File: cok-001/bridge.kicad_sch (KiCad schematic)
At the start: 40 parts, among them U7301 CXD9208GP

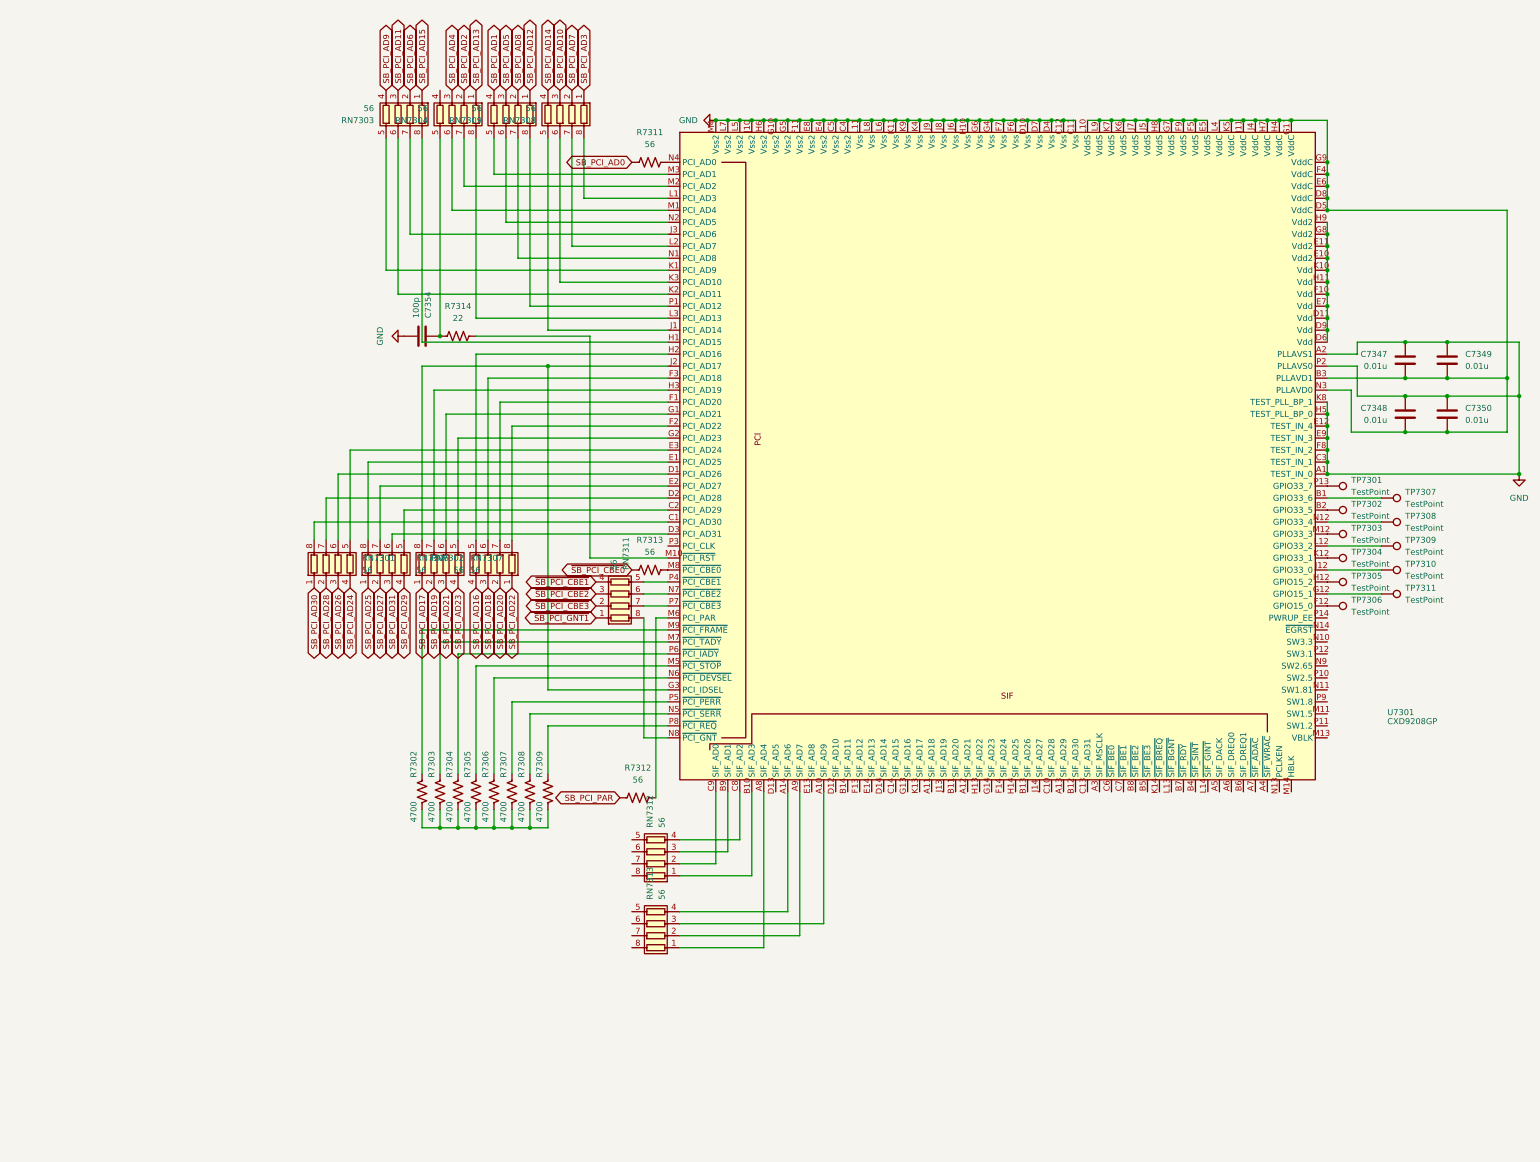
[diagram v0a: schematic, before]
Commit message: add some stupid n channel mosfet
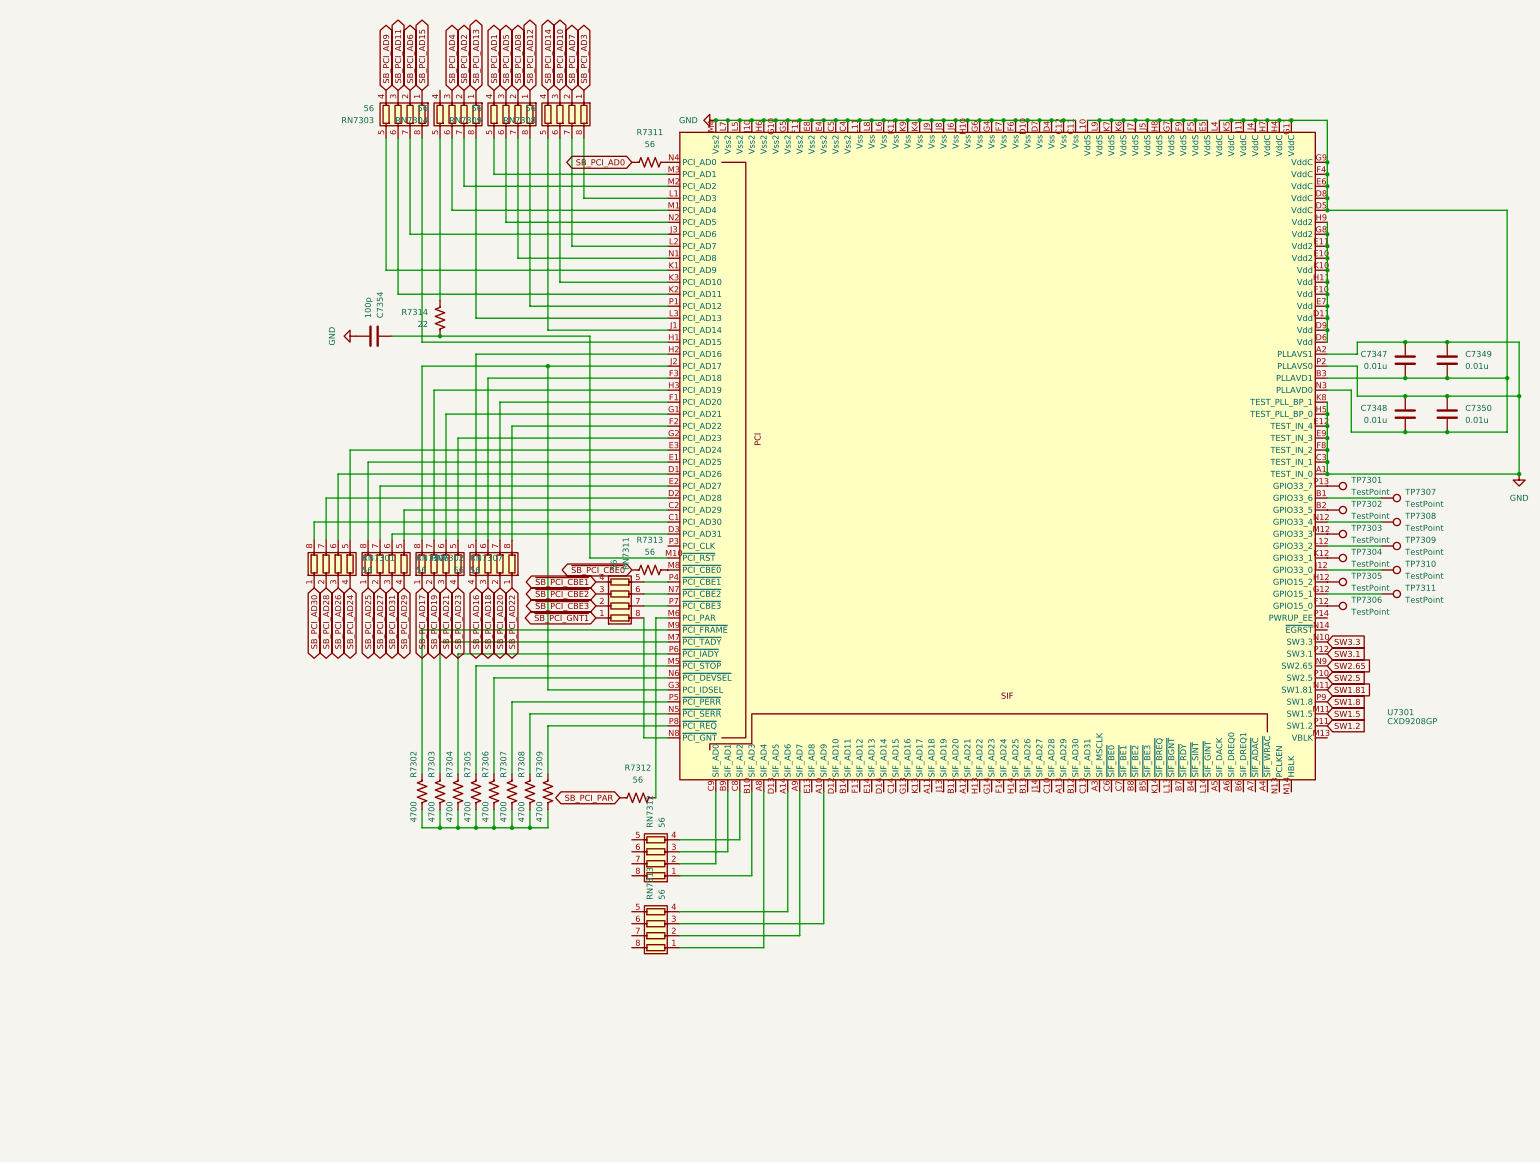
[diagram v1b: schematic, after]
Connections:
- net at C7354.1, R7314.1: now also U7301.M10 (~{PCI_RST}); no longer RN7304.5 (R4.2)
- net at R7314.2: now also RN7304.5 (R4.2); no longer U7301.M10 (~{PCI_RST})
- net SW1.5: now reaches U7301.M11 (SW1.5)
- net SW3.3: now reaches U7301.N10 (SW3.3)
- net SW1.81: now reaches U7301.N11 (SW1.81)
- net SW2.65: now reaches U7301.N9 (SW2.65)
- net SW2.5: now reaches U7301.P10 (SW2.5)
- net SW1.2: now reaches U7301.P11 (SW1.2)
- net SW3.1: now reaches U7301.P12 (SW3.1)
- net SW1.8: now reaches U7301.P9 (SW1.8)
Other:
- moved on the sheet: C7354, R7314
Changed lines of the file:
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@@
 	)
 	(junction
+		(at 48.26 69.85)
+		(diameter 0)
+		(color 0 0 0 0)
+	)
+	(junction
 		(at 152.4 24.13)
 		(diameter 0)
@@
 	)
 	(junction
-		(at 48.26 69.85)
-		(diameter 0)
-		(color 0 0 0 0)
-	)
-	(junction
 		(at 165.1 24.13)
 		(diameter 0)
@@
 	(wire
 		(pts
+			(xy 48.26 62.23) (xy 48.26 27.94)
+		)
+		(stroke
+			(width 0)
+			(type default)
+		)
+	)
+	(wire
+		(pts
 			(xy 129.54 194.31) (xy 99.06 194.31)
 		)
@@
 	(wire
 		(pts
+			(xy 38.1 69.85) (xy 48.26 69.85)
+		)
+		(stroke
+			(width 0)
+			(type default)
+		)
+	)
+	(wire
+		(pts
 			(xy 160.02 24.13) (xy 162.56 24.13)
 		)
@@
 	(wire
 		(pts
-			(xy 80.01 69.85) (xy 55.88 69.85)
-		)
-		(stroke
-			(width 0)
-			(type default)
-		)
-	)
-	(wire
-		(pts
 			(xy 236.22 60.96) (xy 236.22 63.5)
 		)
@@
 	(wire
 		(pts
-			(xy 48.26 27.94) (xy 48.26 69.85)
+			(xy 48.26 69.85) (xy 80.01 69.85)
 		)
 		(stroke
@@
 		)
 	)
+	(global_label "SW1.81"
+		(shape input)
+		(at 236.22 144.78 0)
+		(fields_autoplaced yes)
+		(effects
+			(font
+				(size 1.27 1.27)
+			)
+			(justify left)
+		)
+		(property "Intersheetrefs" "${INTERSHEET_REFS}"
+			(at 246.0994 144.78 0)
+			(effects
+				(font
+					(size 1.27 1.27)
+				)
+				(justify left)
+				(hide yes)
+			)
+		)
+	)
 	(global_label "~{SB_PCI_CBE2}"
 		(shape bidirectional)
@@
 		)
 	)
+	(global_label "SW1.2"
+		(shape input)
+		(at 236.22 152.4 0)
+		(fields_autoplaced yes)
+		(effects
+			(font
+				(size 1.27 1.27)
+			)
+			(justify left)
+		)
+		(property "Intersheetrefs" "${INTERSHEET_REFS}"
+			(at 244.8899 152.4 0)
+			(effects
+				(font
+					(size 1.27 1.27)
+				)
+				(justify left)
+				(hide yes)
+			)
+		)
+	)
+	(global_label "SW2.65"
+		(shape input)
+		(at 236.22 139.7 0)
+		(fields_autoplaced yes)
+		(effects
+			(font
+				(size 1.27 1.27)
+			)
+			(justify left)
+		)
+		(property "Intersheetrefs" "${INTERSHEET_REFS}"
+			(at 246.0994 139.7 0)
+			(effects
+				(font
+					(size 1.27 1.27)
+				)
+				(justify left)
+				(hide yes)
+			)
+		)
+	)
 	(global_label "SB_PCI_AD4"
 		(shape bidirectional)
@@
 		)
 	)
+	(global_label "SW1.8"
+		(shape input)
+		(at 236.22 147.32 0)
+		(fields_autoplaced yes)
+		(effects
+			(font
+				(size 1.27 1.27)
+			)
+			(justify left)
+		)
+		(property "Intersheetrefs" "${INTERSHEET_REFS}"
+			(at 244.8899 147.32 0)
+			(effects
+				(font
+					(size 1.27 1.27)
+				)
+				(justify left)
+				(hide yes)
+			)
+		)
+	)
 	(global_label "SB_PCI_AD7"
 		(shape bidirectional)
@@
 		)
 	)
+	(global_label "SW3.1"
+		(shape input)
+		(at 236.22 137.16 0)
+		(fields_autoplaced yes)
+		(effects
+			(font
+				(size 1.27 1.27)
+			)
+			(justify left)
+		)
+		(property "Intersheetrefs" "${INTERSHEET_REFS}"
+			(at 244.8899 137.16 0)
+			(effects
+				(font
+					(size 1.27 1.27)
+				)
+				(justify left)
+				(hide yes)
+			)
+		)
+	)
 	(global_label "SB_PCI_AD12"
 		(shape bidirectional)
@@
 		)
 	)
+	(global_label "SW3.3"
+		(shape input)
+		(at 236.22 134.62 0)
+		(fields_autoplaced yes)
+		(effects
+			(font
+				(size 1.27 1.27)
+			)
+			(justify left)
+		)
+		(property "Intersheetrefs" "${INTERSHEET_REFS}"
+			(at 244.8899 134.62 0)
+			(effects
+				(font
+					(size 1.27 1.27)
+				)
+				(justify left)
+				(hide yes)
+			)
+		)
+	)
+	(global_label "SW1.5"
+		(shape input)
+		(at 236.22 149.86 0)
+		(fields_autoplaced yes)
+		(effects
+			(font
+				(size 1.27 1.27)
+			)
+			(justify left)
+		)
+		(property "Intersheetrefs" "${INTERSHEET_REFS}"
+			(at 244.8899 149.86 0)
+			(effects
+				(font
+					(size 1.27 1.27)
+				)
+				(justify left)
+				(hide yes)
+			)
+		)
+	)
 	(global_label "SB_PCI_AD26"
 		(shape bidirectional)
@@
 		)
 	)
+	(global_label "SW2.5"
+		(shape input)
+		(at 236.22 142.24 0)
+		(fields_autoplaced yes)
+		(effects
+			(font
+				(size 1.27 1.27)
+			)
+			(justify left)
+		)
+		(property "Intersheetrefs" "${INTERSHEET_REFS}"
+			(at 244.8899 142.24 0)
+			(effects
+				(font
+					(size 1.27 1.27)
+				)
+				(justify left)
+				(hide yes)
+			)
+		)
+	)
 	(symbol
 		(lib_id "Connector:TestPoint")
@@
 	(symbol
 		(lib_id "Device:C")
-		(at 44.45 69.85 270)
+		(at 34.29 69.85 270)
 		(unit 1)
 		(exclude_from_sim no)
@@
 		(dnp no)
 		(property "Reference" "C7354"
-			(at 45.7201 66.04 0)
+			(at 35.5601 66.04 0)
 			(effects
 				(font
@@
 		)
 		(property "Value" "100p"
-			(at 43.1801 66.04 0)
+			(at 33.0201 66.04 0)
 			(effects
 				(font
@@
 		)
 		(property "Footprint" "Capacitor_SMD:C_0402_1005Metric"
-			(at 40.64 70.8152 0)
+			(at 30.48 70.8152 0)
 			(effects
 				(font
@@
 		)
 		(property "Datasheet" "~"
-			(at 44.45 69.85 0)
+			(at 34.29 69.85 0)
 			(effects
 				(font
@@
 		)
 		(property "Description" "Unpolarized capacitor"
-			(at 44.45 69.85 0)
+			(at 34.29 69.85 0)
 			(effects
 				(font
@@
 	(symbol
 		(lib_id "Device:R_US")
-		(at 52.07 69.85 90)
+		(at 48.26 66.04 0)
+		(mirror x)
 		(unit 1)
 		(exclude_from_sim no)
@@
 		(on_board yes)
 		(dnp no)
-		(fields_autoplaced yes)
 		(property "Reference" "R7314"
-			(at 52.07 63.5 90)
+			(at 45.72 64.7699 0)
 			(effects
 				(font
 					(size 1.27 1.27)
 				)
+				(justify right)
 			)
 		)
 		(property "Value" "22"
-			(at 52.07 66.04 90)
+			(at 45.72 67.3099 0)
 			(effects
 				(font
 					(size 1.27 1.27)
 				)
+				(justify right)
 			)
 		)
 		(property "Footprint" "Resistor_SMD:R_0402_1005Metric"
-			(at 52.324 68.834 90)
+			(at 49.276 65.786 90)
 			(effects
 				(font
@@
 		)
 		(property "Datasheet" "~"
-			(at 52.07 69.85 0)
+			(at 48.26 66.04 0)
 			(effects
 				(font
@@
 		)
 		(property "Description" "Resistor, US symbol"
-			(at 52.07 69.85 0)
+			(at 48.26 66.04 0)
 			(effects
 				(font
@@
 	(symbol
 		(lib_id "power:GND")
-		(at 40.64 69.85 270)
+		(at 30.48 69.85 270)
 		(unit 1)
 		(exclude_from_sim no)
@@
 		(fields_autoplaced yes)
 		(property "Reference" "#PWR0503"
-			(at 34.29 69.85 0)
+			(at 24.13 69.85 0)
 			(effects
 				(font
@@
 		)
 		(property "Value" "GND"
-			(at 35.56 69.85 0)
+			(at 25.4 69.85 0)
 			(effects
 				(font
@@
 		)
 		(property "Footprint" ""
-			(at 40.64 69.85 0)
+			(at 30.48 69.85 0)
 			(effects
 				(font
@@
 		)
 		(property "Datasheet" ""
-			(at 40.64 69.85 0)
+			(at 30.48 69.85 0)
 			(effects
 				(font
@@
 		)
 		(property "Description" "Power symbol creates a global label with name \"GND\" , ground"
-			(at 40.64 69.85 0)
+			(at 30.48 69.85 0)
 			(effects
 				(font

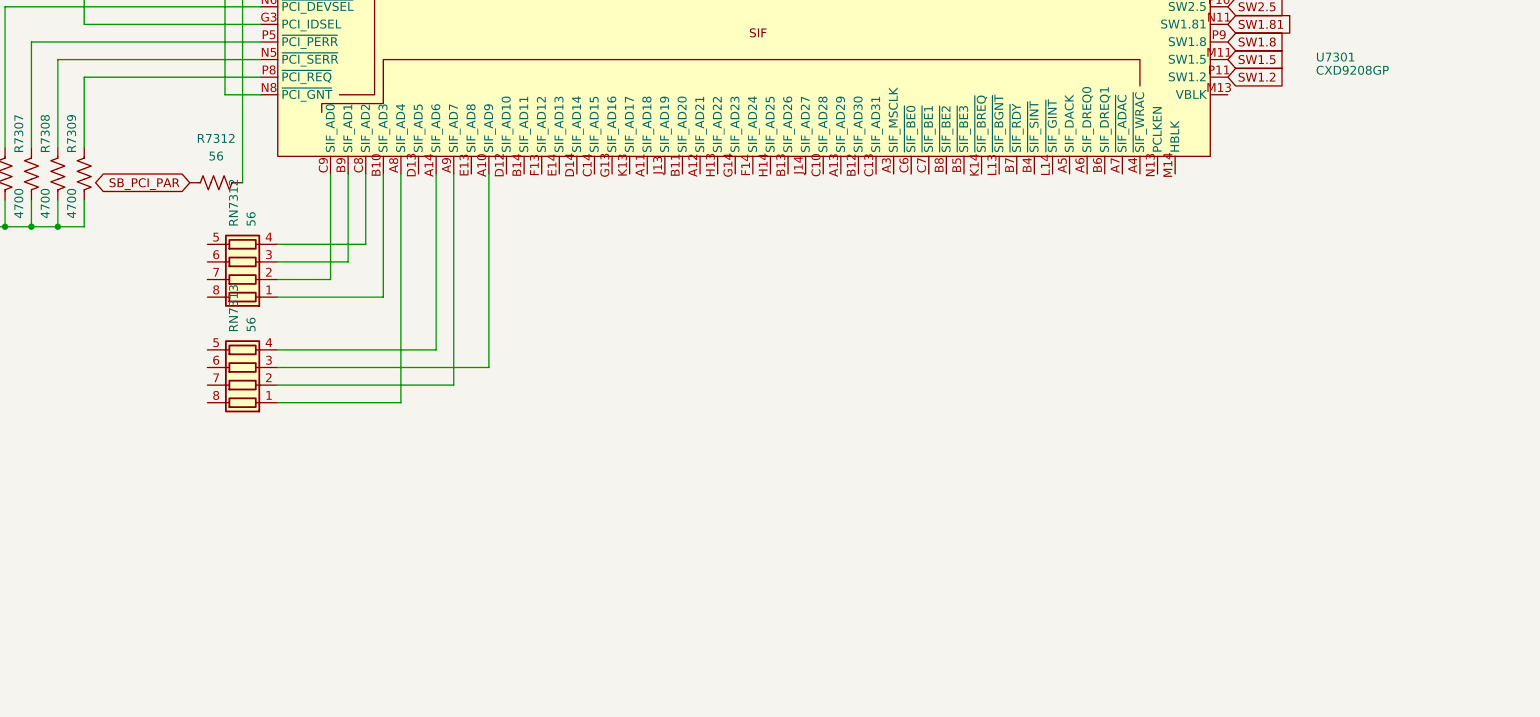
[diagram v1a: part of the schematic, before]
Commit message: bridge sif
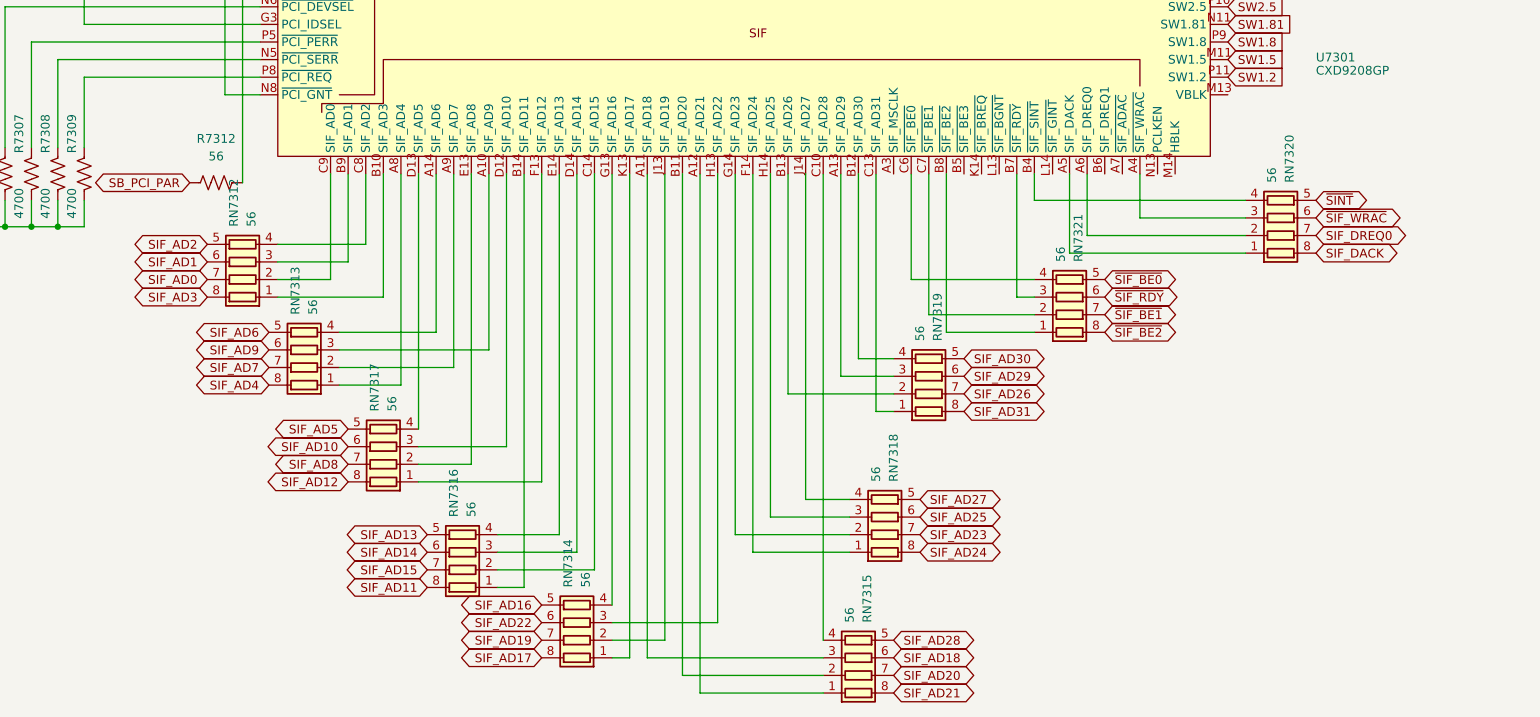
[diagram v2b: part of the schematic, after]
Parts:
- added RN7314, RN7315, RN7316, RN7317, RN7318, RN7319, RN7320, RN7321: 56, Resistor_SMD:R_Array_Convex_4x0402, symbol Device:R_Pack04
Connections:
- net SIF_AD6: now reaches RN7313.5 (R4.2)
- net SIF_AD9: now reaches RN7313.6 (R3.2)
- net SIF_AD7: now reaches RN7313.7 (R2.2)
- net SIF_AD4: now reaches RN7313.8 (R1.2)
- net SIF_AD2: now reaches RN7312.5 (R4.2)
- net SIF_AD1: now reaches RN7312.6 (R3.2)
- net SIF_AD0: now reaches RN7312.7 (R2.2)
- net SIF_AD3: now reaches RN7312.8 (R1.2)
- net at U7301.A11 (SIF_AD18): now also RN7315.3 (R3.1)
- net at U7301.A12 (SIF_AD21): now also RN7315.1 (R1.1)
- net at U7301.A13 (SIF_AD29): now also RN7319.3 (R3.1)
- net at U7301.A4 (~{SIF_WRAC}): now also RN7320.3 (R3.1)
- net at U7301.A5 (SIF_DACK): now also RN7320.1 (R1.1)
- net at U7301.A6 (SIF_DREQ0): now also RN7320.2 (R2.1)
- net at U7301.B11 (SIF_AD20): now also RN7315.2 (R2.1)
- net at U7301.B12 (SIF_AD30): now also RN7319.4 (R4.1)
- net at U7301.B13 (SIF_AD26): now also RN7319.2 (R2.1)
- net at U7301.B14 (SIF_AD11): now also RN7316.1 (R1.1)
- net at U7301.B4 (~{SIF_SINT}): now also RN7320.4 (R4.1)
- net at U7301.B7 (~{SIF_RDY}): now also RN7321.3 (R3.1)
- net at U7301.B8 (~{SIF_BE2}): now also RN7321.1 (R1.1)
- net at U7301.C10 (SIF_AD28): now also RN7315.4 (R4.1)
- net at U7301.C13 (SIF_AD31): now also RN7319.1 (R1.1)
- net at U7301.C14 (SIF_AD15): now also RN7316.2 (R2.1)
- net at U7301.C6 (~{SIF_BE0}): now also RN7321.4 (R4.1)
- net at U7301.C7 (~{SIF_BE1}): now also RN7321.2 (R2.1)
- net at U7301.D12 (SIF_AD10): now also RN7317.3 (R3.1)
- net at U7301.D13 (SIF_AD5): now also RN7317.4 (R4.1)
- net at U7301.D14 (SIF_AD14): now also RN7316.3 (R3.1)
- net at U7301.E13 (SIF_AD8): now also RN7317.2 (R2.1)
- net at U7301.E14 (SIF_AD13): now also RN7316.4 (R4.1)
- net at U7301.F13 (SIF_AD12): now also RN7317.1 (R1.1)
- net at U7301.F14 (SIF_AD24): now also RN7318.1 (R1.1)
- net at U7301.G13 (SIF_AD16): now also RN7314.4 (R4.1)
- net at U7301.G14 (SIF_AD23): now also RN7318.2 (R2.1)
- net at U7301.H13 (SIF_AD22): now also RN7314.3 (R3.1)
- net at U7301.H14 (SIF_AD25): now also RN7318.3 (R3.1)
- net at U7301.J13 (SIF_AD19): now also RN7314.2 (R2.1)
- net at U7301.J14 (SIF_AD27): now also RN7318.4 (R4.1)
- net at U7301.K13 (SIF_AD17): now also RN7314.1 (R1.1)
- new net SIF_AD10: RN7317.6 (R3.2)
- new net SIF_AD11: RN7316.8 (R1.2)
- new net SIF_AD12: RN7317.8 (R1.2)
- new net SIF_AD13: RN7316.5 (R4.2)
- new net SIF_AD14: RN7316.6 (R3.2)
- new net SIF_AD15: RN7316.7 (R2.2)
- new net SIF_AD16: RN7314.5 (R4.2)
- new net SIF_AD17: RN7314.8 (R1.2)
- new net SIF_AD18: RN7315.6 (R3.2)
- new net SIF_AD19: RN7314.7 (R2.2)
- new net SIF_AD20: RN7315.7 (R2.2)
- new net SIF_AD21: RN7315.8 (R1.2)
- new net SIF_AD22: RN7314.6 (R3.2)
- new net SIF_AD23: RN7318.7 (R2.2)
- new net SIF_AD24: RN7318.8 (R1.2)
- new net SIF_AD25: RN7318.6 (R3.2)
- new net SIF_AD26: RN7319.7 (R2.2)
- new net SIF_AD27: RN7318.5 (R4.2)
- new net SIF_AD28: RN7315.5 (R4.2)
- new net SIF_AD29: RN7319.6 (R3.2)
- new net SIF_AD30: RN7319.5 (R4.2)
- new net SIF_AD31: RN7319.8 (R1.2)
- new net SIF_AD5: RN7317.5 (R4.2)
- new net SIF_AD8: RN7317.7 (R2.2)
- new net SIF_DACK: RN7320.8 (R1.2)
- new net SIF_DREQ0: RN7320.7 (R2.2)
- new net ~{SIF_BE0}: RN7321.5 (R4.2)
- new net ~{SIF_BE1}: RN7321.7 (R2.2)
- new net ~{SIF_BE2}: RN7321.8 (R1.2)
- new net ~{SIF_RDY}: RN7321.6 (R3.2)
- new net ~{SIF_WRAC}: RN7320.6 (R3.2)
- new net ~{SINT}: RN7320.5 (R4.2)
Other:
- moved on the sheet: RN7313
